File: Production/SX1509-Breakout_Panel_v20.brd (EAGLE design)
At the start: 142.7 x 121.4 mm, 483 parts, among them U1 SX1509, U10 SX1509, U11 SX1509, U12 SX1509, U13 SX1509, U14 SX1509, U15 SX1509, U2 SX1509, U3 SX1509, U4 SX1509, U5 SX1509, U6 SX1509, U7 SX1509, U8 SX1509, U9 SX1509

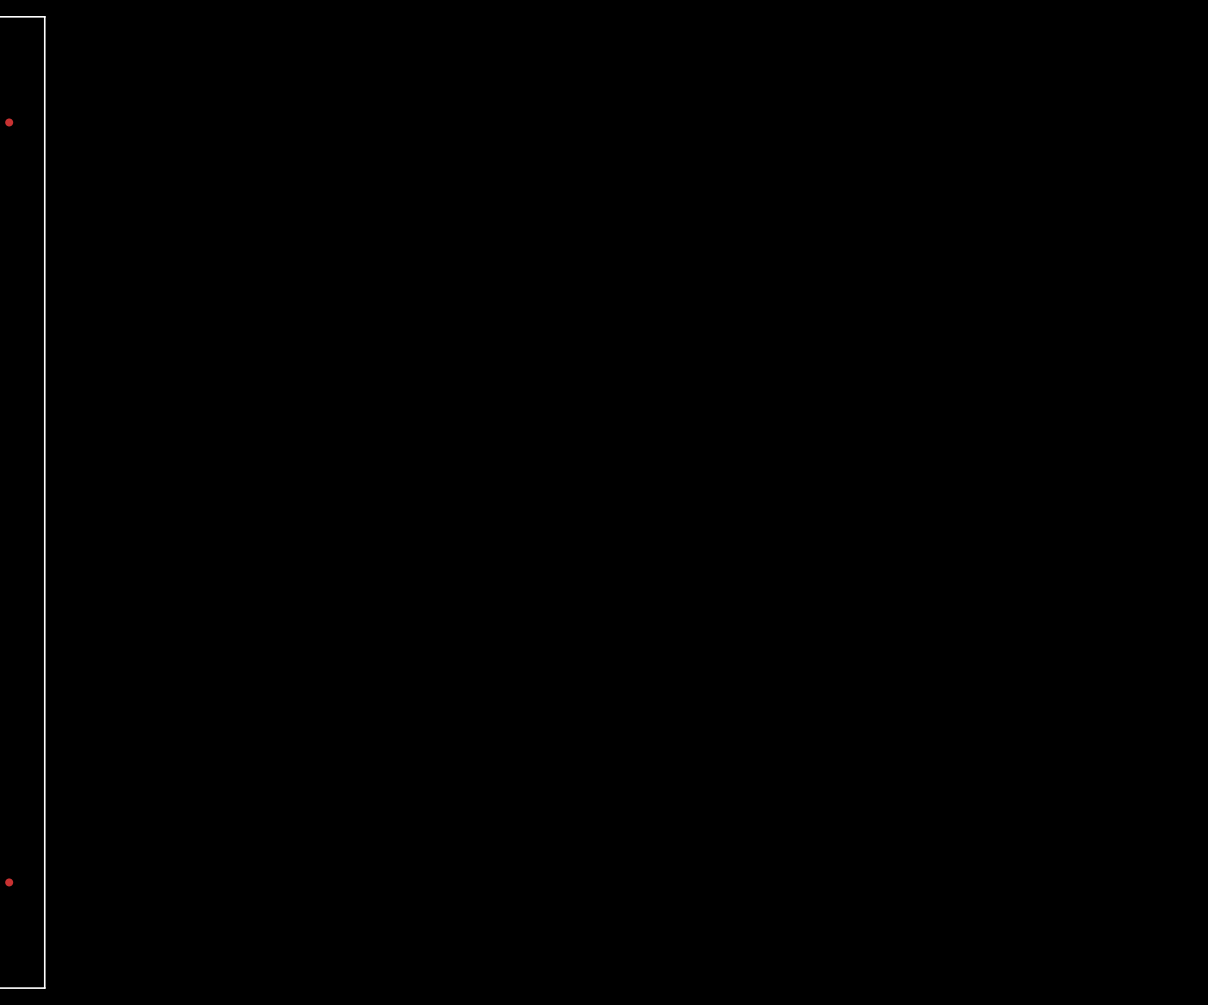
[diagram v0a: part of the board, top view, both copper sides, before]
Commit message: made panel v20 larger
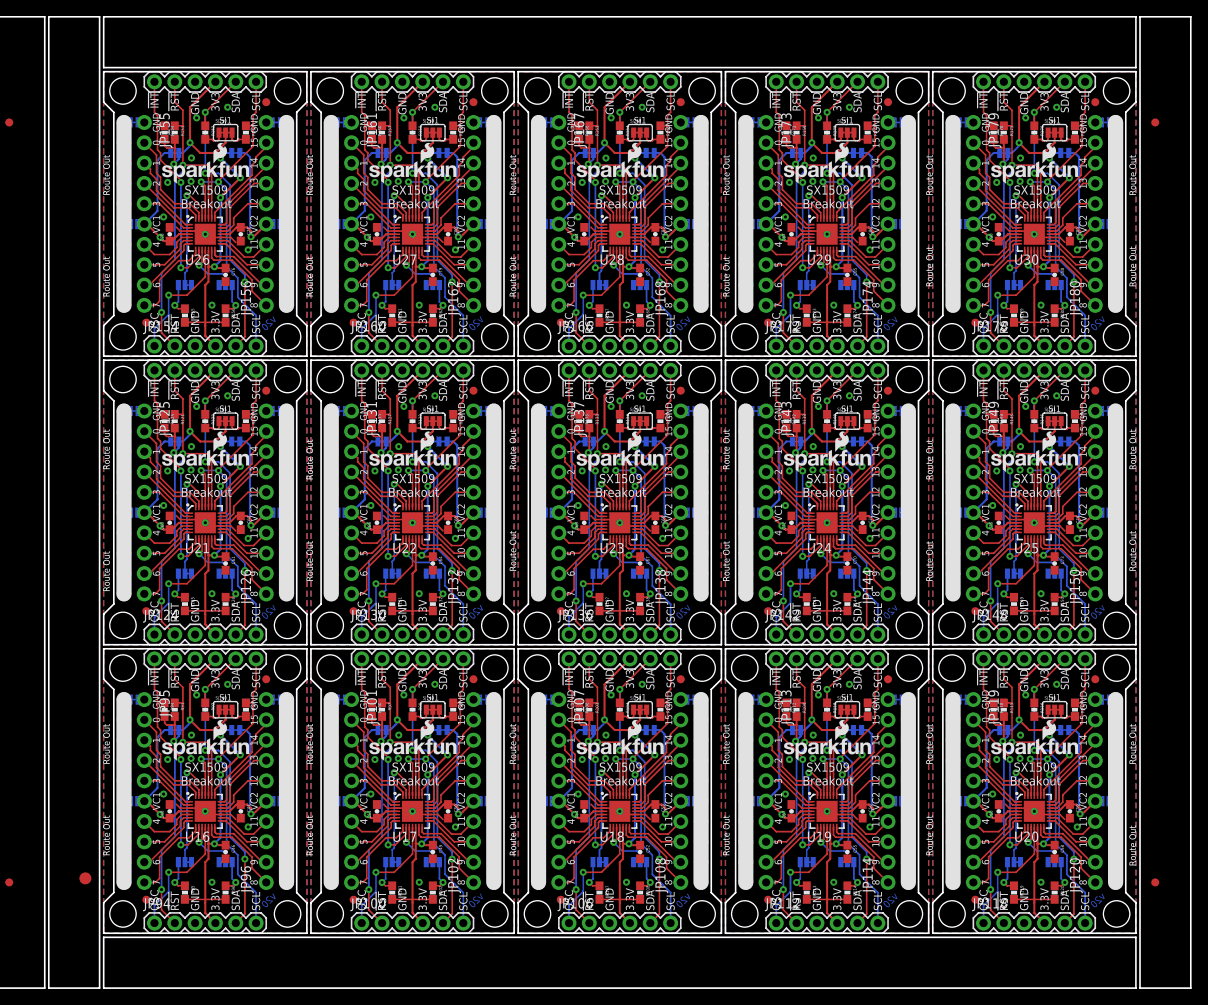
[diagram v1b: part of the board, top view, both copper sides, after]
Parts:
- added C46, C47, C48, C49, C50, C51, C52, C53, C54, C55, C56, C57, C58, C59, C60, C61, C62, C63, C64, C65, C66, C67, C68, C69, C70, C71, C72, C73, C74, C75, C76, C77, C78, C79, C80, C81, C82, C83, C84, C85, C86, C87, C88, C89, C90: 0.1uF, SparkFun-Capacitors:0603-CAP
- added E$2, E$3: (no value), SparkFun-Aesthetics:FIDUCIAL-1X2
- added E$6: (no value), SparkFun-Retired:FIDUCIAL-1.5X3
- added JP100, JP105, JP106, JP111, JP112, JP117, JP118, JP123, JP124, JP129, JP130, JP135, JP136, JP141, JP142, JP147, JP148, JP153, JP154, JP159, JP160, JP165, JP166, JP171, JP172, JP177, JP178, JP93, JP94, JP99: (no value), SparkFun-Connectors:1X06
- added JP101, JP102, JP107, JP108, JP113, JP114, JP119, JP120, JP125, JP126, JP131, JP132, JP137, JP138, JP143, JP144, JP149, JP150, JP155, JP156, JP161, JP162, JP167, JP168, JP173, JP174, JP179, JP180, JP95, JP96: (no value), SparkFun-Connectors:2X10_ROUND_NOSILK
- added JP103, JP104, JP109, JP110, JP115, JP116, JP121, JP122, JP127, JP128, JP133, JP134, JP139, JP140, JP145, JP146, JP151, JP152, JP157, JP158, JP163, JP164, JP169, JP170, JP175, JP176, JP91, JP92, JP97, JP98: FIDUCIAL1X2, SparkFun:FIDUCIAL-1X2
- added LOGO46, LOGO49, LOGO52, LOGO55, LOGO58, LOGO61, LOGO64, LOGO67, LOGO70, LOGO73, LOGO76, LOGO79, LOGO82, LOGO85, LOGO88: OSHW-LOGOS, SparkFun-Aesthetics:OSHW-LOGO-S
- added LOGO47, LOGO50, LOGO53, LOGO56, LOGO59, LOGO62, LOGO65, LOGO68, LOGO71, LOGO74, LOGO77, LOGO80, LOGO83, LOGO86, LOGO89: SFE_LOGO_FLAME.1_INCH, SparkFun-Aesthetics:SFE_LOGO_FLAME_.1
- added LOGO48, LOGO51, LOGO54, LOGO57, LOGO60, LOGO63, LOGO66, LOGO69, LOGO72, LOGO75, LOGO78, LOGO81, LOGO84, LOGO87, LOGO90: SFE_LOGO_NAME_FLAME.1_INCH, SparkFun-Aesthetics:SFE_LOGO_NAME_FLAME_.1
- added R100, R101, R102, R103, R104, R105, R106, R107, R108, R109, R110, R111, R112, R113, R114, R115, R116, R117, R118, R119, R120, R121, R122, R123, R124, R125, R126, R127, R128, R129, R130, R131, R132, R133, R134, R135, R136, R137, R138, R139, R140, R141, R142, R143, R144, R145, R146, R147, R148, R149, R150, R151, R152, R153, R154, R155, R156, R157, R158, R159, R160, R161, R162, R163, R164, R165, R166, R167, R168, R169, R170, R171, R172, R173, R174, R175, R176, R177, R178, R179, R180, R91, R92, R93, R94, R95, R96, R97, R98, R99: 10K, SparkFun-Resistors:0603-RES
- added SJ136, SJ145, SJ154, SJ163, SJ172, SJ181, SJ190, SJ199, SJ208, SJ217, SJ226, SJ235, SJ244, SJ253, SJ262: VCC1-3.3V, SparkFun-Passives:PAD-JUMPER-2-NC_BY_TRACE_YES_SILK
- added SJ137, SJ146, SJ155, SJ164, SJ173, SJ182, SJ191, SJ200, SJ209, SJ218, SJ227, SJ236, SJ245, SJ254, SJ263: VCC2-3.3V, SparkFun-Passives:PAD-JUMPER-2-NC_BY_TRACE_YES_SILK
- added SJ138, SJ139, SJ147, SJ148, SJ156, SJ157, SJ165, SJ166, SJ174, SJ175, SJ183, SJ184, SJ192, SJ193, SJ201, SJ202, SJ210, SJ211, SJ219, SJ220, SJ228, SJ229, SJ237, SJ238, SJ246, SJ247, SJ255, SJ256, SJ264, SJ265: (no value), SparkFun-Passives:PAD-JUMPER-3-2OF3_NC_BY_TRACE_YES_SILK_FULL_BOX
- added SJ140, SJ149, SJ158, SJ167, SJ176, SJ185, SJ194, SJ203, SJ212, SJ221, SJ230, SJ239, SJ248, SJ257, SJ266: (no value), SparkFun-Passives:PAD-JUMPER-3-3OF3_NC_BY_TRACE_YES_SILK_FULL_BOX
- added SJ141, SJ150, SJ159, SJ168, SJ177, SJ186, SJ195, SJ204, SJ213, SJ222, SJ231, SJ240, SJ249, SJ258, SJ267: A-VCC1, SparkFun-Passives:PAD-JUMPER-2-NO_NO_SILK
- added SJ142, SJ151, SJ160, SJ169, SJ178, SJ187, SJ196, SJ205, SJ214, SJ223, SJ232, SJ241, SJ250, SJ259, SJ268: B-VCC2, SparkFun-Passives:PAD-JUMPER-2-NO_NO_SILK
- added SJ143, SJ144, SJ152, SJ153, SJ161, SJ162, SJ170, SJ171, SJ179, SJ180, SJ188, SJ189, SJ197, SJ198, SJ206, SJ207, SJ215, SJ216, SJ224, SJ225, SJ233, SJ234, SJ242, SJ243, SJ251, SJ252, SJ260, SJ261, SJ269, SJ270: GND, SparkFun-Passives:PAD-JUMPER-2-NC_BY_TRACE_NO_SILK
- added STANDOFF100, STANDOFF101, STANDOFF102, STANDOFF103, STANDOFF104, STANDOFF105, STANDOFF106, STANDOFF107, STANDOFF108, STANDOFF109, STANDOFF110, STANDOFF111, STANDOFF112, STANDOFF113, STANDOFF114, STANDOFF115, STANDOFF116, STANDOFF117, STANDOFF118, STANDOFF119, STANDOFF120, STANDOFF61, STANDOFF62, STANDOFF63, STANDOFF64, STANDOFF65, STANDOFF66, STANDOFF67, STANDOFF68, STANDOFF69, STANDOFF70, STANDOFF71, STANDOFF72, STANDOFF73, STANDOFF74, STANDOFF75, STANDOFF76, STANDOFF77, STANDOFF78, STANDOFF79, STANDOFF80, STANDOFF81, STANDOFF82, STANDOFF83, STANDOFF84, STANDOFF85, STANDOFF86, STANDOFF87, STANDOFF88, STANDOFF89, STANDOFF90, STANDOFF91, STANDOFF92, STANDOFF93, STANDOFF94, STANDOFF95, STANDOFF96, STANDOFF97, STANDOFF98, STANDOFF99: STAND-OFF, SparkFun-Electromechanical:STAND-OFF
- added U16, U17, U18, U19, U20, U21, U22, U23, U24, U25, U26, U27, U28, U29, U30: SX1509, SparkFun-DigitalIC:QFN-28
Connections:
- new net !INT15: JP93.1, R94.1, U16.9
- new net !INT16: JP99.1, R100.1, U17.9
- new net !INT17: JP105.1, R106.1, U18.9
- new net !INT18: JP111.1, R112.1, U19.9
- new net !INT19: JP117.1, R118.1, U20.9
- new net !INT20: JP123.1, R124.1, U21.9
- new net !INT21: JP129.1, R130.1, U22.9
- new net !INT22: JP135.1, R136.1, U23.9
- new net !INT23: JP141.1, R142.1, U24.9
- new net !INT24: JP147.1, R148.1, U25.9
- new net !INT25: JP153.1, R154.1, U26.9
- new net !INT26: JP159.1, R160.1, U27.9
- new net !INT27: JP165.1, R166.1, U28.9
- new net !INT28: JP171.1, R172.1, U29.9
- new net !INT29: JP177.1, R178.1, U30.9
- new net !RESET15: JP93.2, JP94.2, R91.1, U16.23
- new net !RESET16: JP100.2, JP99.2, R97.1, U17.23
- new net !RESET17: JP105.2, JP106.2, R103.1, U18.23
- new net !RESET18: JP111.2, JP112.2, R109.1, U19.23
- new net !RESET19: JP117.2, JP118.2, R115.1, U20.23
- new net !RESET20: JP123.2, JP124.2, R121.1, U21.23
- new net !RESET21: JP129.2, JP130.2, R127.1, U22.23
- new net !RESET22: JP135.2, JP136.2, R133.1, U23.23
- new net !RESET23: JP141.2, JP142.2, R139.1, U24.23
- new net !RESET24: JP147.2, JP148.2, R145.1, U25.23
- new net !RESET25: JP153.2, JP154.2, R151.1, U26.23
- new net !RESET26: JP159.2, JP160.2, R157.1, U27.23
- new net !RESET27: JP165.2, JP166.2, R163.1, U28.23
- new net !RESET28: JP171.2, JP172.2, R169.1, U29.23
- new net !RESET29: JP177.2, JP178.2, R175.1, U30.23
- new net 240: JP96.2, U16.13
- new net 241: JP96.4, U16.14
- new net 242: JP96.6, U16.15
- new net 243: JP96.8, U16.16
- new net 244: JP96.12, U16.19
- new net 245: JP96.14, U16.20
- new net 246: JP96.16, U16.21
- new net 247: JP96.18, U16.22
- new net 248: JP95.4, U16.27
- new net 249: JP95.6, U16.28
- new net 250: JP95.8, U16.1
- new net 251: JP95.10, U16.2
- new net 252: JP95.14, U16.5
- new net 253: JP95.16, U16.6
- new net 254: JP95.18, U16.7
- new net 255: JP95.20, U16.8
- new net 256: JP102.2, U17.13
- new net 257: JP102.4, U17.14
- new net 258: JP102.6, U17.15
- new net 259: JP102.8, U17.16
- new net 260: JP102.12, U17.19
- new net 261: JP102.14, U17.20
- new net 262: JP102.16, U17.21
- new net 263: JP102.18, U17.22
- new net 264: JP101.4, U17.27
- new net 265: JP101.6, U17.28
- new net 266: JP101.8, U17.1
- new net 267: JP101.10, U17.2
- new net 268: JP101.14, U17.5
- new net 269: JP101.16, U17.6
- new net 270: JP101.18, U17.7
- new net 271: JP101.20, U17.8
- new net 272: JP108.2, U18.13
- new net 273: JP108.4, U18.14
- new net 274: JP108.6, U18.15
- new net 275: JP108.8, U18.16
- new net 276: JP108.12, U18.19
- new net 277: JP108.14, U18.20
- new net 278: JP108.16, U18.21
- new net 279: JP108.18, U18.22
- new net 280: JP107.4, U18.27
- new net 281: JP107.6, U18.28
- new net 282: JP107.8, U18.1
- new net 283: JP107.10, U18.2
- new net 284: JP107.14, U18.5
- new net 285: JP107.16, U18.6
- new net 286: JP107.18, U18.7
- new net 287: JP107.20, U18.8
- new net 288: JP114.2, U19.13
- new net 289: JP114.4, U19.14
- new net 290: JP114.6, U19.15
- new net 291: JP114.8, U19.16
- new net 292: JP114.12, U19.19
- new net 293: JP114.14, U19.20
- new net 294: JP114.16, U19.21
- new net 295: JP114.18, U19.22
- new net 296: JP113.4, U19.27
- new net 297: JP113.6, U19.28
- new net 298: JP113.8, U19.1
- new net 299: JP113.10, U19.2
- new net 3.3V15: C46.1, JP93.4, JP94.4, R91.2, R94.2, R95.2, R96.2, SJ136.2, SJ137.2, SJ140.2, U16.12
- new net 3.3V16: C49.1, JP100.4, JP99.4, R100.2, R101.2, R102.2, R97.2, SJ145.2, SJ146.2, SJ149.2, U17.12
- new net 3.3V17: C52.1, JP105.4, JP106.4, R103.2, R106.2, R107.2, R108.2, SJ154.2, SJ155.2, SJ158.2, U18.12
- new net 3.3V18: C55.1, JP111.4, JP112.4, R109.2, R112.2, R113.2, R114.2, SJ163.2, SJ164.2, SJ167.2, U19.12
- new net 3.3V19: C58.1, JP117.4, JP118.4, R115.2, R118.2, R119.2, R120.2, SJ172.2, SJ173.2, SJ176.2, U20.12
- new net 3.3V20: C61.1, JP123.4, JP124.4, R121.2, R124.2, R125.2, R126.2, SJ181.2, SJ182.2, SJ185.2, U21.12
- new net 3.3V21: C64.1, JP129.4, JP130.4, R127.2, R130.2, R131.2, R132.2, SJ190.2, SJ191.2, SJ194.2, U22.12
- new net 3.3V22: C67.1, JP135.4, JP136.4, R133.2, R136.2, R137.2, R138.2, SJ199.2, SJ200.2, SJ203.2, U23.12
- new net 3.3V23: C70.1, JP141.4, JP142.4, R139.2, R142.2, R143.2, R144.2, SJ208.2, SJ209.2, SJ212.2, U24.12
- new net 3.3V24: C73.1, JP147.4, JP148.4, R145.2, R148.2, R149.2, R150.2, SJ217.2, SJ218.2, SJ221.2, U25.12
- new net 3.3V25: C76.1, JP153.4, JP154.4, R151.2, R154.2, R155.2, R156.2, SJ226.2, SJ227.2, SJ230.2, U26.12
- new net 3.3V26: C79.1, JP159.4, JP160.4, R157.2, R160.2, R161.2, R162.2, SJ235.2, SJ236.2, SJ239.2, U27.12
- new net 3.3V27: C82.1, JP165.4, JP166.4, R163.2, R166.2, R167.2, R168.2, SJ244.2, SJ245.2, SJ248.2, U28.12
- new net 3.3V28: C85.1, JP171.4, JP172.4, R169.2, R172.2, R173.2, R174.2, SJ253.2, SJ254.2, SJ257.2, U29.12
- new net 3.3V29: C88.1, JP177.4, JP178.4, R175.2, R178.2, R179.2, R180.2, SJ262.2, SJ263.2, SJ266.2, U30.12
- new net 300: JP113.14, U19.5
- new net 301: JP113.16, U19.6
- new net 302: JP113.18, U19.7
- new net 303: JP113.20, U19.8
- new net 304: JP120.2, U20.13
- new net 305: JP120.4, U20.14
- new net 306: JP120.6, U20.15
- new net 307: JP120.8, U20.16
- new net 308: JP120.12, U20.19
- new net 309: JP120.14, U20.20
- new net 310: JP120.16, U20.21
- new net 311: JP120.18, U20.22
- new net 312: JP119.4, U20.27
- new net 313: JP119.6, U20.28
- new net 314: JP119.8, U20.1
- new net 315: JP119.10, U20.2
- new net 316: JP119.14, U20.5
- new net 317: JP119.16, U20.6
- new net 318: JP119.18, U20.7
- new net 319: JP119.20, U20.8
- new net 320: JP126.2, U21.13
- new net 321: JP126.4, U21.14
- new net 322: JP126.6, U21.15
- new net 323: JP126.8, U21.16
- new net 324: JP126.12, U21.19
- new net 325: JP126.14, U21.20
- new net 326: JP126.16, U21.21
- new net 327: JP126.18, U21.22
- new net 328: JP125.4, U21.27
- new net 329: JP125.6, U21.28
- new net 330: JP125.8, U21.1
- new net 331: JP125.10, U21.2
- new net 332: JP125.14, U21.5
- new net 333: JP125.16, U21.6
- new net 334: JP125.18, U21.7
- new net 335: JP125.20, U21.8
- new net 336: JP132.2, U22.13
- new net 337: JP132.4, U22.14
- new net 338: JP132.6, U22.15
- new net 339: JP132.8, U22.16
- new net 340: JP132.12, U22.19
- new net 341: JP132.14, U22.20
- new net 342: JP132.16, U22.21
- new net 343: JP132.18, U22.22
- new net 344: JP131.4, U22.27
- new net 345: JP131.6, U22.28
- new net 346: JP131.8, U22.1
- new net 347: JP131.10, U22.2
- new net 348: JP131.14, U22.5
- new net 349: JP131.16, U22.6
- new net 350: JP131.18, U22.7
- new net 351: JP131.20, U22.8
- new net 352: JP138.2, U23.13
- new net 353: JP138.4, U23.14
- new net 354: JP138.6, U23.15
- new net 355: JP138.8, U23.16
- new net 356: JP138.12, U23.19
- new net 357: JP138.14, U23.20
- new net 358: JP138.16, U23.21
- new net 359: JP138.18, U23.22
- new net 360: JP137.4, U23.27
- new net 361: JP137.6, U23.28
- new net 362: JP137.8, U23.1
- new net 363: JP137.10, U23.2
- new net 364: JP137.14, U23.5
- new net 365: JP137.16, U23.6
- new net 366: JP137.18, U23.7
- new net 367: JP137.20, U23.8
- new net 368: JP144.2, U24.13
- new net 369: JP144.4, U24.14
- new net 370: JP144.6, U24.15
- new net 371: JP144.8, U24.16
- new net 372: JP144.12, U24.19
- new net 373: JP144.14, U24.20
- new net 374: JP144.16, U24.21
- new net 375: JP144.18, U24.22
- new net 376: JP143.4, U24.27
- new net 377: JP143.6, U24.28
- new net 378: JP143.8, U24.1
- new net 379: JP143.10, U24.2
- new net 380: JP143.14, U24.5
- new net 381: JP143.16, U24.6
- new net 382: JP143.18, U24.7
- new net 383: JP143.20, U24.8
- new net 384: JP150.2, U25.13
- new net 385: JP150.4, U25.14
- new net 386: JP150.6, U25.15
- new net 387: JP150.8, U25.16
- new net 388: JP150.12, U25.19
- new net 389: JP150.14, U25.20
- new net 390: JP150.16, U25.21
- new net 391: JP150.18, U25.22
- new net 392: JP149.4, U25.27
- new net 393: JP149.6, U25.28
- new net 394: JP149.8, U25.1
- new net 395: JP149.10, U25.2
- new net 396: JP149.14, U25.5
- new net 397: JP149.16, U25.6
- new net 398: JP149.18, U25.7
- new net 399: JP149.20, U25.8
- new net 400: JP156.2, U26.13
- new net 401: JP156.4, U26.14
- new net 402: JP156.6, U26.15
- new net 403: JP156.8, U26.16
- new net 404: JP156.12, U26.19
- new net 405: JP156.14, U26.20
- new net 406: JP156.16, U26.21
- new net 407: JP156.18, U26.22
- new net 408: JP155.4, U26.27
- new net 409: JP155.6, U26.28
- new net 410: JP155.8, U26.1
- new net 411: JP155.10, U26.2
- new net 412: JP155.14, U26.5
- new net 413: JP155.16, U26.6
- new net 414: JP155.18, U26.7
- new net 415: JP155.20, U26.8
- new net 416: JP162.2, U27.13
- new net 417: JP162.4, U27.14
- new net 418: JP162.6, U27.15
- new net 419: JP162.8, U27.16
- new net 420: JP162.12, U27.19
- new net 421: JP162.14, U27.20
- new net 422: JP162.16, U27.21
- new net 423: JP162.18, U27.22
- new net 424: JP161.4, U27.27
- new net 425: JP161.6, U27.28
- new net 426: JP161.8, U27.1
- new net 427: JP161.10, U27.2
- new net 428: JP161.14, U27.5
- new net 429: JP161.16, U27.6
- new net 430: JP161.18, U27.7
- new net 431: JP161.20, U27.8
- new net 432: JP168.2, U28.13
- new net 433: JP168.4, U28.14
- new net 434: JP168.6, U28.15
- new net 435: JP168.8, U28.16
- new net 436: JP168.12, U28.19
- new net 437: JP168.14, U28.20
- new net 438: JP168.16, U28.21
- new net 439: JP168.18, U28.22
- new net 440: JP167.4, U28.27
- new net 441: JP167.6, U28.28
- new net 442: JP167.8, U28.1
- new net 443: JP167.10, U28.2
- new net 444: JP167.14, U28.5
- new net 445: JP167.16, U28.6
- new net 446: JP167.18, U28.7
- new net 447: JP167.20, U28.8
- new net 448: JP174.2, U29.13
- new net 449: JP174.4, U29.14
- new net 450: JP174.6, U29.15
- new net 451: JP174.8, U29.16
- new net 452: JP174.12, U29.19
- new net 453: JP174.14, U29.20
- new net 454: JP174.16, U29.21
- new net 455: JP174.18, U29.22
- new net 456: JP173.4, U29.27
- new net 457: JP173.6, U29.28
- new net 458: JP173.8, U29.1
- new net 459: JP173.10, U29.2
- new net 460: JP173.14, U29.5
- new net 461: JP173.16, U29.6
- new net 462: JP173.18, U29.7
- new net 463: JP173.20, U29.8
- new net 464: JP180.2, U30.13
- new net 465: JP180.4, U30.14
- new net 466: JP180.6, U30.15
- new net 467: JP180.8, U30.16
- new net 468: JP180.12, U30.19
- new net 469: JP180.14, U30.20
- new net 470: JP180.16, U30.21
- new net 471: JP180.18, U30.22
- new net 472: JP179.4, U30.27
- new net 473: JP179.6, U30.28
- new net 474: JP179.8, U30.1
- new net 475: JP179.10, U30.2
- new net 476: JP179.14, U30.5
- new net 477: JP179.16, U30.6
- new net 478: JP179.18, U30.7
- new net 479: JP179.20, U30.8
- new net ADDR30: SJ139.2, U16.26
- new net ADDR31: SJ138.2, U16.10
- new net ADDR32: SJ148.2, U17.26
- new net ADDR33: SJ147.2, U17.10
- new net ADDR34: SJ157.2, U18.26
- new net ADDR35: SJ156.2, U18.10
- new net ADDR36: SJ166.2, U19.26
- new net ADDR37: SJ165.2, U19.10
- new net ADDR38: SJ175.2, U20.26
- new net ADDR39: SJ174.2, U20.10
- new net ADDR40: SJ184.2, U21.26
- new net ADDR41: SJ183.2, U21.10
- new net ADDR42: SJ193.2, U22.26
- new net ADDR43: SJ192.2, U22.10
- new net ADDR44: SJ202.2, U23.26
- new net ADDR45: SJ201.2, U23.10
- new net ADDR46: SJ211.2, U24.26
- new net ADDR47: SJ210.2, U24.10
- new net ADDR48: SJ220.2, U25.26
- new net ADDR49: SJ219.2, U25.10
- new net ADDR50: SJ229.2, U26.26
- new net ADDR51: SJ228.2, U26.10
- new net ADDR52: SJ238.2, U27.26
- new net ADDR53: SJ237.2, U27.10
- new net ADDR54: SJ247.2, U28.26
- new net ADDR55: SJ246.2, U28.10
- new net ADDR56: SJ256.2, U29.26
- new net ADDR57: SJ255.2, U29.10
- new net ADDR58: SJ265.2, U30.26
- new net ADDR59: SJ264.2, U30.10
- new net GND15: C46.2, C47.2, C48.2, JP93.3, JP94.3, JP95.2, JP96.20, SJ138.3, SJ139.3, SJ143.1, SJ144.1, U16.17, U16.29, U16.3
- new net GND16: C49.2, C50.2, C51.2, JP100.3, JP101.2, JP102.20, JP99.3, SJ147.3, SJ148.3, SJ152.1, SJ153.1, U17.17, U17.29, U17.3
- new net GND17: C52.2, C53.2, C54.2, JP105.3, JP106.3, JP107.2, JP108.20, SJ156.3, SJ157.3, SJ161.1, SJ162.1, U18.17, U18.29, U18.3
- new net GND18: C55.2, C56.2, C57.2, JP111.3, JP112.3, JP113.2, JP114.20, SJ165.3, SJ166.3, SJ170.1, SJ171.1, U19.17, U19.29, U19.3
- new net GND19: C58.2, C59.2, C60.2, JP117.3, JP118.3, JP119.2, JP120.20, SJ174.3, SJ175.3, SJ179.1, SJ180.1, U20.17, U20.29, U20.3
- new net GND20: C61.2, C62.2, C63.2, JP123.3, JP124.3, JP125.2, JP126.20, SJ183.3, SJ184.3, SJ188.1, SJ189.1, U21.17, U21.29, U21.3
- new net GND21: C64.2, C65.2, C66.2, JP129.3, JP130.3, JP131.2, JP132.20, SJ192.3, SJ193.3, SJ197.1, SJ198.1, U22.17, U22.29, U22.3
- new net GND22: C67.2, C68.2, C69.2, JP135.3, JP136.3, JP137.2, JP138.20, SJ201.3, SJ202.3, SJ206.1, SJ207.1, U23.17, U23.29, U23.3
- new net GND23: C70.2, C71.2, C72.2, JP141.3, JP142.3, JP143.2, JP144.20, SJ210.3, SJ211.3, SJ215.1, SJ216.1, U24.17, U24.29, U24.3
- new net GND24: C73.2, C74.2, C75.2, JP147.3, JP148.3, JP149.2, JP150.20, SJ219.3, SJ220.3, SJ224.1, SJ225.1, U25.17, U25.29, U25.3
- new net GND25: C76.2, C77.2, C78.2, JP153.3, JP154.3, JP155.2, JP156.20, SJ228.3, SJ229.3, SJ233.1, SJ234.1, U26.17, U26.29, U26.3
- new net GND26: C79.2, C80.2, C81.2, JP159.3, JP160.3, JP161.2, JP162.20, SJ237.3, SJ238.3, SJ242.1, SJ243.1, U27.17, U27.29, U27.3
- new net GND27: C82.2, C83.2, C84.2, JP165.3, JP166.3, JP167.2, JP168.20, SJ246.3, SJ247.3, SJ251.1, SJ252.1, U28.17, U28.29, U28.3
- new net GND28: C85.2, C86.2, C87.2, JP171.3, JP172.3, JP173.2, JP174.20, SJ255.3, SJ256.3, SJ260.1, SJ261.1, U29.17, U29.29, U29.3
- new net GND29: C88.2, C89.2, C90.2, JP177.3, JP178.3, JP179.2, JP180.20, SJ264.3, SJ265.3, SJ269.1, SJ270.1, U30.17, U30.29, U30.3
- new net N$100: JP120.1, JP120.11, JP120.13, JP120.15, JP120.17, JP120.19, JP120.3, JP120.5, JP120.7, JP120.9, SJ178.1, SJ179.2
- new net N$101: R123.2, SJ185.3
- new net N$102: R122.2, SJ185.1
- new net N$103: R125.1, SJ184.1
- new net N$104: R126.1, SJ183.1
- new net N$105: JP126.1, JP126.11, JP126.13, JP126.15, JP126.17, JP126.19, JP126.3, JP126.5, JP126.7, JP126.9, SJ187.1, SJ188.2
- new net N$106: R129.2, SJ194.3
- new net N$107: R128.2, SJ194.1
- new net N$108: R131.1, SJ193.1
- new net N$109: R132.1, SJ192.1
- new net N$110: JP132.1, JP132.11, JP132.13, JP132.15, JP132.17, JP132.19, JP132.3, JP132.5, JP132.7, JP132.9, SJ196.1, SJ197.2
- new net N$111: R135.2, SJ203.3
- new net N$112: R134.2, SJ203.1
- new net N$113: R137.1, SJ202.1
- new net N$114: R138.1, SJ201.1
- new net N$115: JP138.1, JP138.11, JP138.13, JP138.15, JP138.17, JP138.19, JP138.3, JP138.5, JP138.7, JP138.9, SJ205.1, SJ206.2
- new net N$116: R141.2, SJ212.3
- new net N$117: R140.2, SJ212.1
- new net N$118: R143.1, SJ211.1
- new net N$119: R144.1, SJ210.1
- new net N$120: JP144.1, JP144.11, JP144.13, JP144.15, JP144.17, JP144.19, JP144.3, JP144.5, JP144.7, JP144.9, SJ214.1, SJ215.2
- new net N$121: R147.2, SJ221.3
- new net N$122: R146.2, SJ221.1
- new net N$123: R149.1, SJ220.1
- new net N$124: R150.1, SJ219.1
- new net N$125: JP150.1, JP150.11, JP150.13, JP150.15, JP150.17, JP150.19, JP150.3, JP150.5, JP150.7, JP150.9, SJ223.1, SJ224.2
- new net N$126: R153.2, SJ230.3
- new net N$127: R152.2, SJ230.1
- new net N$128: R155.1, SJ229.1
- new net N$129: R156.1, SJ228.1
- new net N$130: JP156.1, JP156.11, JP156.13, JP156.15, JP156.17, JP156.19, JP156.3, JP156.5, JP156.7, JP156.9, SJ232.1, SJ233.2
- new net N$131: R159.2, SJ239.3
- new net N$132: R158.2, SJ239.1
- new net N$133: R161.1, SJ238.1
- new net N$134: R162.1, SJ237.1
- new net N$135: JP162.1, JP162.11, JP162.13, JP162.15, JP162.17, JP162.19, JP162.3, JP162.5, JP162.7, JP162.9, SJ241.1, SJ242.2
- new net N$136: R165.2, SJ248.3
- new net N$137: R164.2, SJ248.1
- new net N$138: R167.1, SJ247.1
- new net N$139: R168.1, SJ246.1
- new net N$140: JP168.1, JP168.11, JP168.13, JP168.15, JP168.17, JP168.19, JP168.3, JP168.5, JP168.7, JP168.9, SJ250.1, SJ251.2
- new net N$141: R171.2, SJ257.3
- new net N$142: R170.2, SJ257.1
- new net N$143: R173.1, SJ256.1
- new net N$144: R174.1, SJ255.1
- new net N$145: JP174.1, JP174.11, JP174.13, JP174.15, JP174.17, JP174.19, JP174.3, JP174.5, JP174.7, JP174.9, SJ259.1, SJ260.2
- new net N$146: R177.2, SJ266.3
- new net N$147: R176.2, SJ266.1
- new net N$148: R179.1, SJ265.1
- new net N$149: R180.1, SJ264.1
- new net N$150: JP180.1, JP180.11, JP180.13, JP180.15, JP180.17, JP180.19, JP180.3, JP180.5, JP180.7, JP180.9, SJ268.1, SJ269.2
- new net N$76: R93.2, SJ140.3
- new net N$77: R92.2, SJ140.1
- new net N$78: R95.1, SJ139.1
- new net N$79: R96.1, SJ138.1
- new net N$80: JP96.1, JP96.11, JP96.13, JP96.15, JP96.17, JP96.19, JP96.3, JP96.5, JP96.7, JP96.9, SJ142.1, SJ143.2
- new net N$81: R99.2, SJ149.3
- new net N$82: R98.2, SJ149.1
- new net N$83: R101.1, SJ148.1
- new net N$84: R102.1, SJ147.1
- new net N$85: JP102.1, JP102.11, JP102.13, JP102.15, JP102.17, JP102.19, JP102.3, JP102.5, JP102.7, JP102.9, SJ151.1, SJ152.2
- new net N$86: R105.2, SJ158.3
- new net N$87: R104.2, SJ158.1
- new net N$88: R107.1, SJ157.1
- new net N$89: R108.1, SJ156.1
- new net N$90: JP108.1, JP108.11, JP108.13, JP108.15, JP108.17, JP108.19, JP108.3, JP108.5, JP108.7, JP108.9, SJ160.1, SJ161.2
- new net N$91: R111.2, SJ167.3
- new net N$92: R110.2, SJ167.1
- new net N$93: R113.1, SJ166.1
- new net N$94: R114.1, SJ165.1
- new net N$95: JP114.1, JP114.11, JP114.13, JP114.15, JP114.17, JP114.19, JP114.3, JP114.5, JP114.7, JP114.9, SJ169.1, SJ170.2
- new net N$96: R117.2, SJ176.3
- new net N$97: R116.2, SJ176.1
- new net N$98: R119.1, SJ175.1
- new net N$99: R120.1, SJ174.1
- new net OSCIO15: JP94.1, U16.11
- new net OSCIO16: JP100.1, U17.11
- new net OSCIO17: JP106.1, U18.11
- new net OSCIO18: JP112.1, U19.11
- new net OSCIO19: JP118.1, U20.11
- new net OSCIO20: JP124.1, U21.11
- new net OSCIO21: JP130.1, U22.11
- new net OSCIO22: JP136.1, U23.11
- new net OSCIO23: JP142.1, U24.11
- new net OSCIO24: JP148.1, U25.11
- new net OSCIO25: JP154.1, U26.11
- new net OSCIO26: JP160.1, U27.11
- new net OSCIO27: JP166.1, U28.11
- new net OSCIO28: JP172.1, U29.11
- new net OSCIO29: JP178.1, U30.11
- new net PWRBUSA15: JP95.1, JP95.11, JP95.13, JP95.15, JP95.17, JP95.19, JP95.3, JP95.5, JP95.7, JP95.9, SJ141.1, SJ144.2
- new net PWRBUSA16: JP101.1, JP101.11, JP101.13, JP101.15, JP101.17, JP101.19, JP101.3, JP101.5, JP101.7, JP101.9, SJ150.1, SJ153.2
- new net PWRBUSA17: JP107.1, JP107.11, JP107.13, JP107.15, JP107.17, JP107.19, JP107.3, JP107.5, JP107.7, JP107.9, SJ159.1, SJ162.2
- new net PWRBUSA18: JP113.1, JP113.11, JP113.13, JP113.15, JP113.17, JP113.19, JP113.3, JP113.5, JP113.7, JP113.9, SJ168.1, SJ171.2
- new net PWRBUSA19: JP119.1, JP119.11, JP119.13, JP119.15, JP119.17, JP119.19, JP119.3, JP119.5, JP119.7, JP119.9, SJ177.1, SJ180.2
- new net PWRBUSA20: JP125.1, JP125.11, JP125.13, JP125.15, JP125.17, JP125.19, JP125.3, JP125.5, JP125.7, JP125.9, SJ186.1, SJ189.2
- new net PWRBUSA21: JP131.1, JP131.11, JP131.13, JP131.15, JP131.17, JP131.19, JP131.3, JP131.5, JP131.7, JP131.9, SJ195.1, SJ198.2
- new net PWRBUSA22: JP137.1, JP137.11, JP137.13, JP137.15, JP137.17, JP137.19, JP137.3, JP137.5, JP137.7, JP137.9, SJ204.1, SJ207.2
- new net PWRBUSA23: JP143.1, JP143.11, JP143.13, JP143.15, JP143.17, JP143.19, JP143.3, JP143.5, JP143.7, JP143.9, SJ213.1, SJ216.2
- new net PWRBUSA24: JP149.1, JP149.11, JP149.13, JP149.15, JP149.17, JP149.19, JP149.3, JP149.5, JP149.7, JP149.9, SJ222.1, SJ225.2
- new net PWRBUSA25: JP155.1, JP155.11, JP155.13, JP155.15, JP155.17, JP155.19, JP155.3, JP155.5, JP155.7, JP155.9, SJ231.1, SJ234.2
- new net PWRBUSA26: JP161.1, JP161.11, JP161.13, JP161.15, JP161.17, JP161.19, JP161.3, JP161.5, JP161.7, JP161.9, SJ240.1, SJ243.2
- new net PWRBUSA27: JP167.1, JP167.11, JP167.13, JP167.15, JP167.17, JP167.19, JP167.3, JP167.5, JP167.7, JP167.9, SJ249.1, SJ252.2
- new net PWRBUSA28: JP173.1, JP173.11, JP173.13, JP173.15, JP173.17, JP173.19, JP173.3, JP173.5, JP173.7, JP173.9, SJ258.1, SJ261.2
- new net PWRBUSA29: JP179.1, JP179.11, JP179.13, JP179.15, JP179.17, JP179.19, JP179.3, JP179.5, JP179.7, JP179.9, SJ267.1, SJ270.2
- new net SCL15: JP93.6, JP94.6, R93.1, U16.25
- new net SCL16: JP100.6, JP99.6, R99.1, U17.25
- new net SCL17: JP105.6, JP106.6, R105.1, U18.25
- new net SCL18: JP111.6, JP112.6, R111.1, U19.25
- new net SCL19: JP117.6, JP118.6, R117.1, U20.25
- new net SCL20: JP123.6, JP124.6, R123.1, U21.25
- new net SCL21: JP129.6, JP130.6, R129.1, U22.25
- new net SCL22: JP135.6, JP136.6, R135.1, U23.25
- new net SCL23: JP141.6, JP142.6, R141.1, U24.25
- new net SCL24: JP147.6, JP148.6, R147.1, U25.25
- new net SCL25: JP153.6, JP154.6, R153.1, U26.25
- new net SCL26: JP159.6, JP160.6, R159.1, U27.25
- new net SCL27: JP165.6, JP166.6, R165.1, U28.25
- new net SCL28: JP171.6, JP172.6, R171.1, U29.25
- new net SCL29: JP177.6, JP178.6, R177.1, U30.25
- new net SDA15: JP93.5, JP94.5, R92.1, U16.24
- new net SDA16: JP100.5, JP99.5, R98.1, U17.24
- new net SDA17: JP105.5, JP106.5, R104.1, U18.24
- new net SDA18: JP111.5, JP112.5, R110.1, U19.24
- new net SDA19: JP117.5, JP118.5, R116.1, U20.24
- new net SDA20: JP123.5, JP124.5, R122.1, U21.24
- new net SDA21: JP129.5, JP130.5, R128.1, U22.24
- new net SDA22: JP135.5, JP136.5, R134.1, U23.24
- new net SDA23: JP141.5, JP142.5, R140.1, U24.24
- new net SDA24: JP147.5, JP148.5, R146.1, U25.24
- new net SDA25: JP153.5, JP154.5, R152.1, U26.24
- new net SDA26: JP159.5, JP160.5, R158.1, U27.24
- new net SDA27: JP165.5, JP166.5, R164.1, U28.24
- new net SDA28: JP171.5, JP172.5, R170.1, U29.24
- new net SDA29: JP177.5, JP178.5, R176.1, U30.24
- new net VCC31: C47.1, JP96.10, SJ137.1, SJ142.2, U16.18
- new net VCC32: C48.1, JP95.12, SJ136.1, SJ141.2, U16.4
- new net VCC33: C50.1, JP102.10, SJ146.1, SJ151.2, U17.18
- new net VCC34: C51.1, JP101.12, SJ145.1, SJ150.2, U17.4
- new net VCC35: C53.1, JP108.10, SJ155.1, SJ160.2, U18.18
- new net VCC36: C54.1, JP107.12, SJ154.1, SJ159.2, U18.4
- new net VCC37: C56.1, JP114.10, SJ164.1, SJ169.2, U19.18
- new net VCC38: C57.1, JP113.12, SJ163.1, SJ168.2, U19.4
- new net VCC39: C59.1, JP120.10, SJ173.1, SJ178.2, U20.18
- new net VCC40: C60.1, JP119.12, SJ172.1, SJ177.2, U20.4
- new net VCC41: C62.1, JP126.10, SJ182.1, SJ187.2, U21.18
- new net VCC42: C63.1, JP125.12, SJ181.1, SJ186.2, U21.4
- new net VCC43: C65.1, JP132.10, SJ191.1, SJ196.2, U22.18
- new net VCC44: C66.1, JP131.12, SJ190.1, SJ195.2, U22.4
- new net VCC45: C68.1, JP138.10, SJ200.1, SJ205.2, U23.18
- new net VCC46: C69.1, JP137.12, SJ199.1, SJ204.2, U23.4
- new net VCC47: C71.1, JP144.10, SJ209.1, SJ214.2, U24.18
- new net VCC48: C72.1, JP143.12, SJ208.1, SJ213.2, U24.4
- new net VCC49: C74.1, JP150.10, SJ218.1, SJ223.2, U25.18
- new net VCC50: C75.1, JP149.12, SJ217.1, SJ222.2, U25.4
- new net VCC51: C77.1, JP156.10, SJ227.1, SJ232.2, U26.18
- new net VCC52: C78.1, JP155.12, SJ226.1, SJ231.2, U26.4
- new net VCC53: C80.1, JP162.10, SJ236.1, SJ241.2, U27.18
- new net VCC54: C81.1, JP161.12, SJ235.1, SJ240.2, U27.4
- new net VCC55: C83.1, JP168.10, SJ245.1, SJ250.2, U28.18
- new net VCC56: C84.1, JP167.12, SJ244.1, SJ249.2, U28.4
- new net VCC57: C86.1, JP174.10, SJ254.1, SJ259.2, U29.18
- new net VCC58: C87.1, JP173.12, SJ253.1, SJ258.2, U29.4
- new net VCC59: C89.1, JP180.10, SJ263.1, SJ268.2, U30.18
- new net VCC60: C90.1, JP179.12, SJ262.1, SJ267.2, U30.4
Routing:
- net 3.3V25: track 0.00 -> 63.7 mm, vias 0 -> 6
- net 3.3V20: track 0.00 -> 63.7 mm, vias 0 -> 6
- net 3.3V15: track 0.00 -> 63.7 mm, vias 0 -> 6
- net 3.3V23: track 0.00 -> 63.7 mm, vias 0 -> 6
- net 3.3V28: track 0.00 -> 63.7 mm, vias 0 -> 6
- net 3.3V21: track 0.00 -> 63.7 mm, vias 0 -> 6
- net 3.3V26: track 0.00 -> 63.7 mm, vias 0 -> 6
- net 3.3V18: track 0.00 -> 63.7 mm, vias 0 -> 6
- net 3.3V16: track 0.00 -> 63.7 mm, vias 0 -> 6
- net 3.3V22: track 0.00 -> 63.7 mm, vias 0 -> 6
- net 3.3V24: track 0.00 -> 63.7 mm, vias 0 -> 6
- net 3.3V27: track 0.00 -> 63.7 mm, vias 0 -> 6
- net 3.3V17: track 0.00 -> 63.7 mm, vias 0 -> 6
- net 3.3V29: track 0.00 -> 63.7 mm, vias 0 -> 6
- net 3.3V19: track 0.00 -> 63.7 mm, vias 0 -> 6
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- added copper zone on layer 1, net GND15
- added copper zone on layer 16, net GND15
- added copper zone on layer 1, net GND16
- added copper zone on layer 16, net GND16
- added copper zone on layer 1, net GND17
- added copper zone on layer 16, net GND17
- added copper zone on layer 1, net GND18
- added copper zone on layer 16, net GND18
- added copper zone on layer 1, net GND19
- added copper zone on layer 16, net GND19
- added copper zone on layer 1, net GND20
- added copper zone on layer 16, net GND20
- added copper zone on layer 1, net GND21
- added copper zone on layer 16, net GND21
- added copper zone on layer 1, net GND22
- added copper zone on layer 16, net GND22
- added copper zone on layer 1, net GND23
- added copper zone on layer 16, net GND23
- added copper zone on layer 1, net GND24
- added copper zone on layer 16, net GND24
- added copper zone on layer 1, net GND25
- added copper zone on layer 16, net GND25
- added copper zone on layer 1, net GND26
- added copper zone on layer 16, net GND26
- added copper zone on layer 1, net GND27
- added copper zone on layer 16, net GND27
- added copper zone on layer 1, net GND28
- added copper zone on layer 16, net GND28
- added copper zone on layer 1, net GND29
- added copper zone on layer 16, net GND29
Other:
- board size 142.7 x 121.4 mm -> 286 x 121.4 mm
